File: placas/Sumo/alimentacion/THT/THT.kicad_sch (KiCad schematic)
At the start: 6 parts

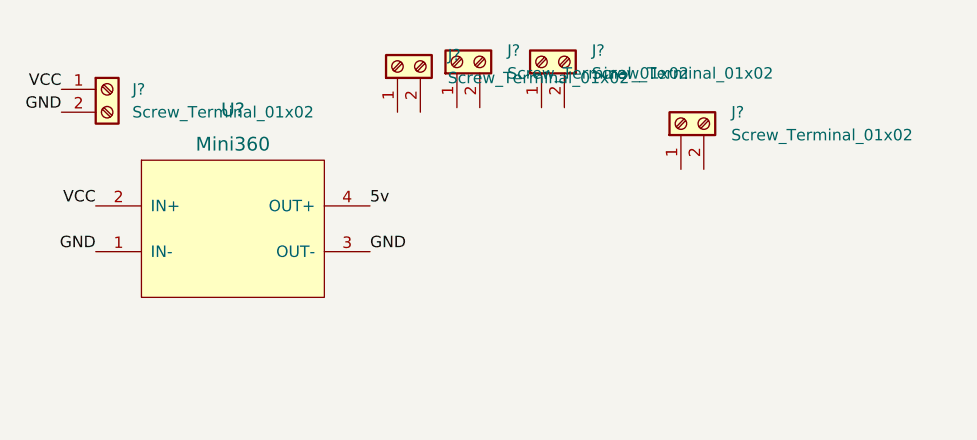
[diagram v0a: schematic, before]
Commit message: fgdgf
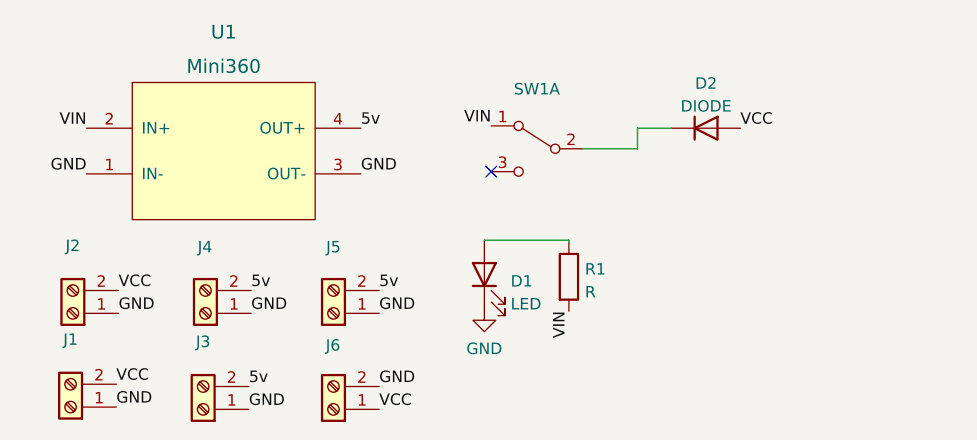
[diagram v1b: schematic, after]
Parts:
- added D1: LED, LED_THT:LED_D3.0mm, symbol Device:LED
- added D2: DIODE, Diode_THT:D_5W_P12.70mm_Horizontal, symbol Simulation_SPICE:DIODE
- added J5: (no value), symbol Connector:Screw_Terminal_01x02
- added R1: R, Resistor_THT:R_Axial_DIN0207_L6.3mm_D2.5mm_P10.16mm_Horizontal, symbol Device:R
- added SW1: (no value), symbol Switch:SW_DPDT_x2
- J1, J2, J3, J4, J6: renamed from J?; value Screw_Terminal_01x02 -> (none)
- gave numbers to parts that had none: 1
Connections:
- net 5v: now also J3.2 (Pin_2), J4.2 (Pin_2), J5.2 (Pin_2)
- net GND: now also J1.1 (Pin_1), J2.1 (Pin_1), J3.1 (Pin_1), J4.1 (Pin_1), D1.1 (K), J5.1 (Pin_1)
- net VCC: now also J1.2 (Pin_2), J2.2 (Pin_2), D2.1 (A); no longer U1.2 (IN+)
- new net: D2.2 (K), SW1.2 (B)
- new net: D1.2 (A), R1.1
- new net VIN: R1.2, SW1.1 (A), U1.2 (IN+)
- no-connect marks 0 -> 1
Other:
- moved on the sheet: J1, J2, J3, J4, J6, U1
